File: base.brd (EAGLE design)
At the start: 100 x 80 mm, 2 parts, among them J1 AS0A626-U2SN-7F, U2 XC7K160TFBG676

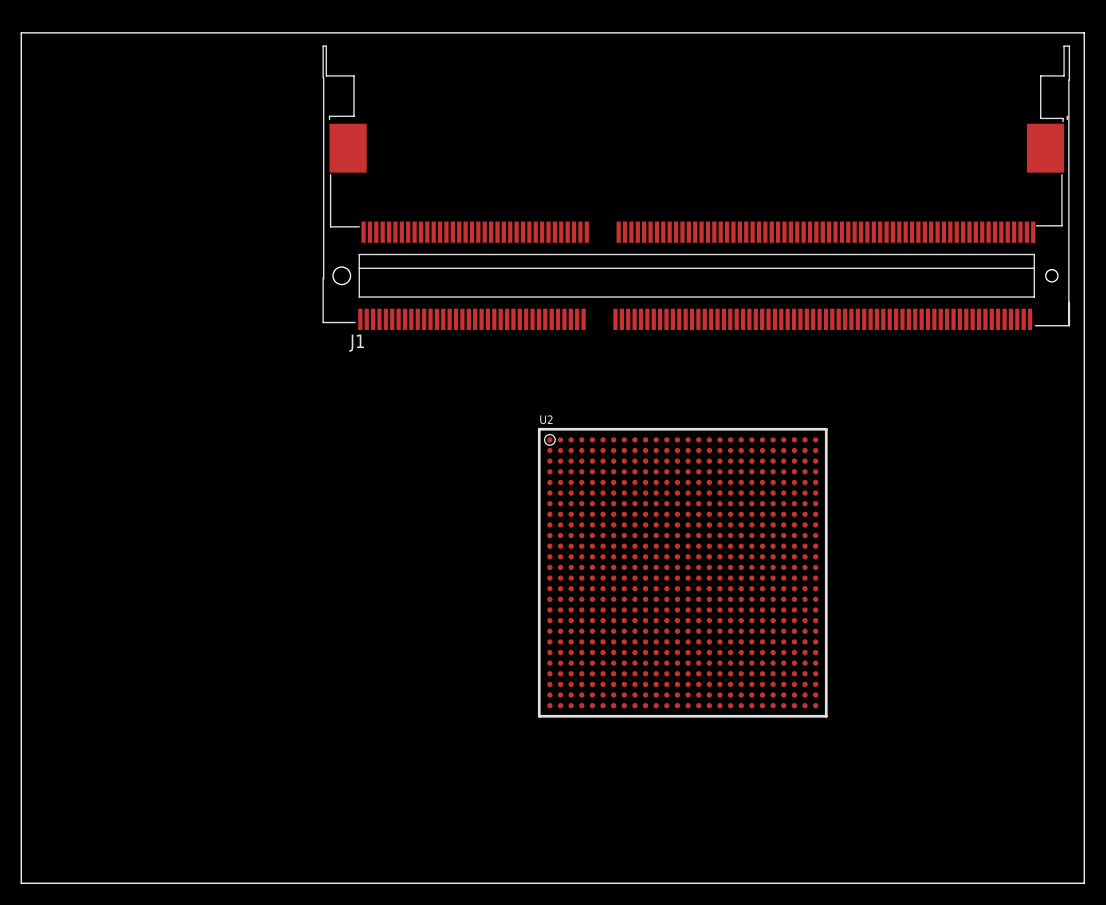
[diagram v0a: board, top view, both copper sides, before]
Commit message: updating for new lib.
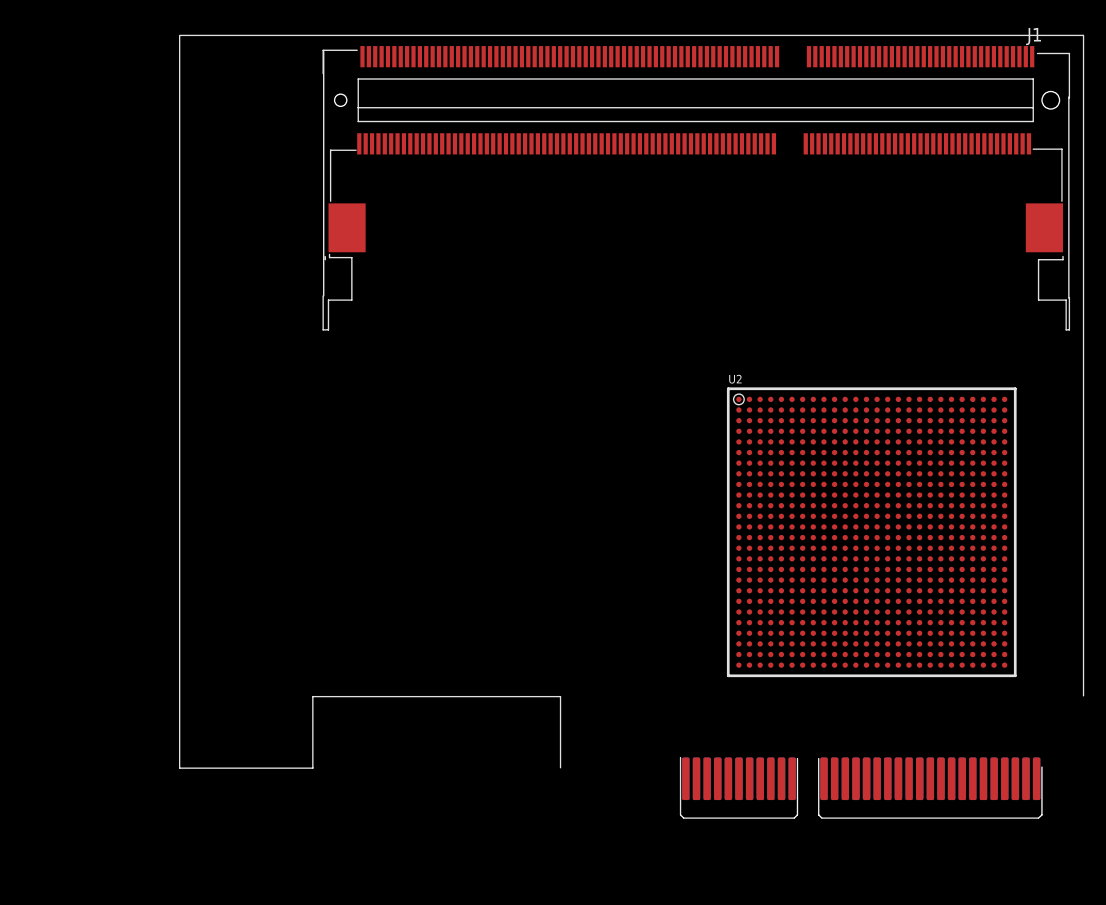
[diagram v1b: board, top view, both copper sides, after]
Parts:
- added U$1: PCIEX4_SMALL_CARD, con-pcie-x4 short card:PCIEX4_SMALL_CARD
- moved U2 18.2 mm to (80.0, 33.0)
- moved J1 16.5 mm to (63.5, 73.7), turned to 180 degrees
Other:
- board size 100 x 80 mm -> 34 x 5.6 mm
